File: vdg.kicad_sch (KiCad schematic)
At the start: 58 parts, among them IC1 74HCT273, IC10 74HCT32, IC11 74LS123N, IC12 LM1889N, IC13 2318, IC15 CD4053, IC2 MC6847, IC3 74HCT00, IC4 74HCT20, IC5 74HCT86, IC6 74HCT393, IC7 74ALS74N, IC8 74HCT393, IC9 74HCT390, Y1 4.433619MHz

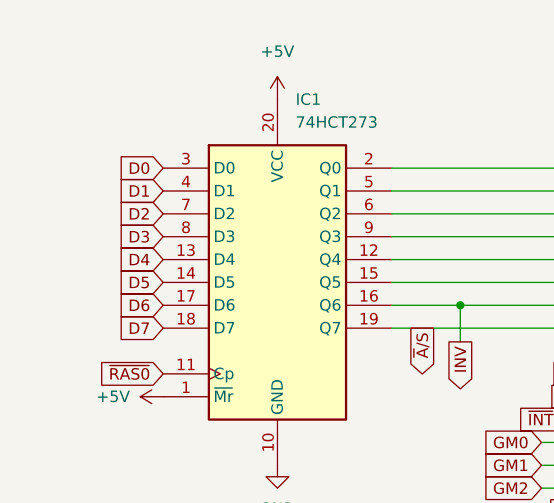
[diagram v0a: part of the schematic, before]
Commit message: rework pcb
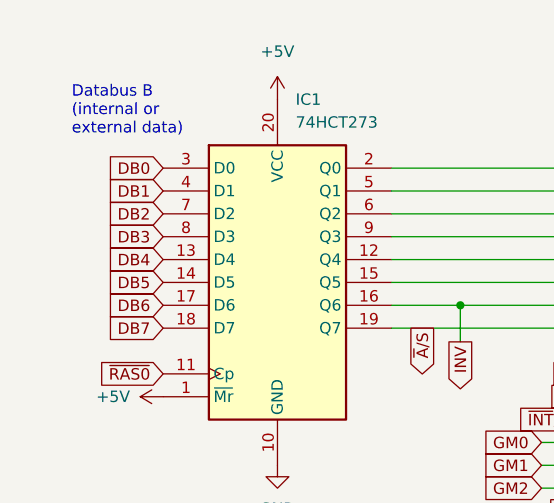
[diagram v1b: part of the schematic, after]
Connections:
- net D0 renamed DB0
- net D1 renamed DB1
- net D2 renamed DB2
- net D3 renamed DB3
- net D4 renamed DB4
- net D5 renamed DB5
- net D6 renamed DB6
- net D7 renamed DB7
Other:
- note added: "Databus B (internal or external data)"
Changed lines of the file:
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@@
+    (effects (font (size 1.27 1.27)) (justify left bottom))
+  )
+  (text "Databus B\n(internal or \nexternal data)" (at 16.51 26.67 0)
     (effects (font (size 1.27 1.27)) (justify left bottom))
   )
@@
     (effects (font (size 1.27 1.27)) (justify left bottom))
   )
-  (global_label "D0" (shape input) (at 26.67 30.226 180) (fields_autoplaced)
-    (effects (font (size 1.27 1.27)) (justify right))
-    (property "Intersheetrefs" "${INTERSHEET_REFS}" (at 21.2053 30.226 0)
+  (global_label "DB0" (shape input) (at 26.67 30.226 180) (fields_autoplaced)
+    (effects (font (size 1.27 1.27)) (justify right))
+    (property "Intersheetrefs" "${INTERSHEET_REFS}" (at 19.9353 30.226 0)
       (effects (font (size 1.27 1.27)) (justify right) hide)
     )
@@
     )
   )
-  (global_label "D6" (shape input) (at 26.67 45.466 180) (fields_autoplaced)
-    (effects (font (size 1.27 1.27)) (justify right))
-    (property "Intersheetrefs" "${INTERSHEET_REFS}" (at 21.2053 45.466 0)
+  (global_label "DB6" (shape input) (at 26.67 45.466 180) (fields_autoplaced)
+    (effects (font (size 1.27 1.27)) (justify right))
+    (property "Intersheetrefs" "${INTERSHEET_REFS}" (at 19.9353 45.466 0)
       (effects (font (size 1.27 1.27)) (justify right) hide)
     )
@@
     )
   )
-  (global_label "D7" (shape input) (at 26.67 48.006 180) (fields_autoplaced)
-    (effects (font (size 1.27 1.27)) (justify right))
-    (property "Intersheetrefs" "${INTERSHEET_REFS}" (at 21.2053 48.006 0)
-      (effects (font (size 1.27 1.27)) (justify right) hide)
-    )
-  )
-  (global_label "D1" (shape input) (at 26.67 32.766 180) (fields_autoplaced)
-    (effects (font (size 1.27 1.27)) (justify right))
-    (property "Intersheetrefs" "${INTERSHEET_REFS}" (at 21.2053 32.766 0)
+  (global_label "DB7" (shape input) (at 26.67 48.006 180) (fields_autoplaced)
+    (effects (font (size 1.27 1.27)) (justify right))
+    (property "Intersheetrefs" "${INTERSHEET_REFS}" (at 19.9353 48.006 0)
+      (effects (font (size 1.27 1.27)) (justify right) hide)
+    )
+  )
+  (global_label "DB1" (shape input) (at 26.67 32.766 180) (fields_autoplaced)
+    (effects (font (size 1.27 1.27)) (justify right))
+    (property "Intersheetrefs" "${INTERSHEET_REFS}" (at 19.9353 32.766 0)
       (effects (font (size 1.27 1.27)) (justify right) hide)
     )
@@
     )
   )
-  (global_label "D5" (shape input) (at 26.67 42.926 180) (fields_autoplaced)
-    (effects (font (size 1.27 1.27)) (justify right))
-    (property "Intersheetrefs" "${INTERSHEET_REFS}" (at 21.2053 42.926 0)
+  (global_label "DB5" (shape input) (at 26.67 42.926 180) (fields_autoplaced)
+    (effects (font (size 1.27 1.27)) (justify right))
+    (property "Intersheetrefs" "${INTERSHEET_REFS}" (at 19.9353 42.926 0)
       (effects (font (size 1.27 1.27)) (justify right) hide)
     )
@@
     )
   )
-  (global_label "D3" (shape input) (at 26.67 37.846 180) (fields_autoplaced)
-    (effects (font (size 1.27 1.27)) (justify right))
-    (property "Intersheetrefs" "${INTERSHEET_REFS}" (at 21.2053 37.846 0)
+  (global_label "DB3" (shape input) (at 26.67 37.846 180) (fields_autoplaced)
+    (effects (font (size 1.27 1.27)) (justify right))
+    (property "Intersheetrefs" "${INTERSHEET_REFS}" (at 19.9353 37.846 0)
       (effects (font (size 1.27 1.27)) (justify right) hide)
     )
@@
     )
   )
-  (global_label "D4" (shape input) (at 26.67 40.386 180) (fields_autoplaced)
-    (effects (font (size 1.27 1.27)) (justify right))
-    (property "Intersheetrefs" "${INTERSHEET_REFS}" (at 21.2053 40.386 0)
+  (global_label "DB4" (shape input) (at 26.67 40.386 180) (fields_autoplaced)
+    (effects (font (size 1.27 1.27)) (justify right))
+    (property "Intersheetrefs" "${INTERSHEET_REFS}" (at 19.9353 40.386 0)
       (effects (font (size 1.27 1.27)) (justify right) hide)
     )
@@
     )
   )
-  (global_label "D2" (shape input) (at 26.67 35.306 180) (fields_autoplaced)
-    (effects (font (size 1.27 1.27)) (justify right))
-    (property "Intersheetrefs" "${INTERSHEET_REFS}" (at 21.2053 35.306 0)
+  (global_label "DB2" (shape input) (at 26.67 35.306 180) (fields_autoplaced)
+    (effects (font (size 1.27 1.27)) (justify right))
+    (property "Intersheetrefs" "${INTERSHEET_REFS}" (at 19.9353 35.306 0)
       (effects (font (size 1.27 1.27)) (justify right) hide)
     )
@@
   )
   (symbol (lib_id "Device:C_Trim_Differential") (at 175.26 95.504 0) (unit 1)
-    (in_bom yes) (on_board yes) (dnp no) (fields_autoplaced)
+    (in_bom yes) (on_board yes) (dnp no)
     (property "Reference" "C7" (at 180.848 94.1069 0)
       (effects (font (size 1.27 1.27)) (justify left))
